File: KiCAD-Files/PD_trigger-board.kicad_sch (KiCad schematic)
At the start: 25 parts, among them J1 USB_C_Receptacle_USB2.0_14P, J10 15V, J11 18V, J2 Conn_01x03, J3 Conn_01x03, J4 VOUT, J5 5V, J6 5V, J7 5V, J8 9V, J9 12V, Q1 AONR21307, U1 HUSB238

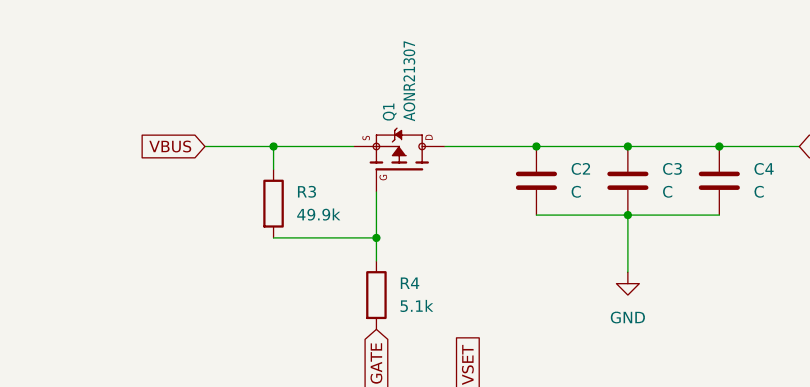
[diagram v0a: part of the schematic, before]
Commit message: Routin fertig
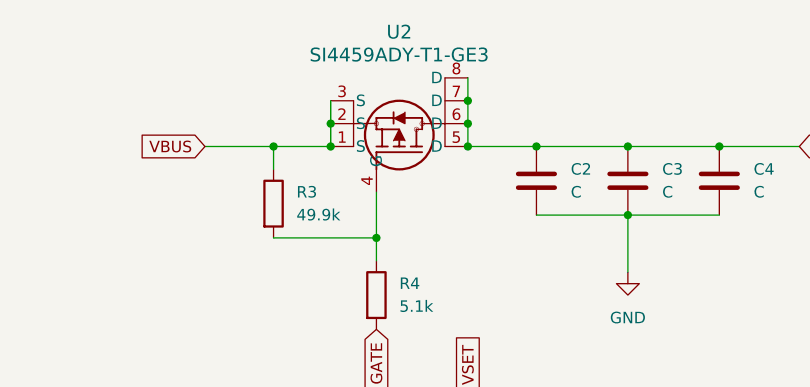
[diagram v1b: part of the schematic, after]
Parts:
- removed Q1: AONR21307, Adafruit HUSB238 USB-C PD Breakout:POWERDI3333, symbol Adafruit HUSB238 USB-C PD Breakout-eagle-import:MOSFET-P-POWERDI3333
- added U2: SI4459ADY-T1-GE3, blinkyparts:SO_ADY-T1-GE3_VIS, symbol SI4459ADY:SI4459ADY-T1-GE3
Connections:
- net VBUS: now also U2.1 (S), U2.2 (S), U2.3 (S)
- net VOUT: now also U2.5 (D), U2.6 (D), U2.7 (D), U2.8 (D)
- net at R3.2, R4.1: now also U2.4 (G)
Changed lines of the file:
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@@
 	(paper "A4")
+	(junction
+		(at 236.22 105.41)
+		(diameter 0)
+		(color 0 0 0 0)
+	)
+	(junction
+		(at 236.22 35.56)
+		(diameter 0)
+		(color 0 0 0 0)
+	)
+	(junction
+		(at 274.32 87.63)
+		(diameter 0)
+		(color 0 0 0 0)
+	)
+	(junction
+		(at 254 35.56)
+		(diameter 0)
+		(color 0 0 0 0)
+	)
+	(junction
+		(at 274.32 96.52)
+		(diameter 0)
+		(color 0 0 0 0)
+	)
+	(junction
+		(at 236.22 87.63)
+		(diameter 0)
+		(color 0 0 0 0)
+	)
+	(junction
+		(at 175.26 138.43)
+		(diameter 0)
+		(color 0 0 0 0)
+	)
+	(junction
+		(at 274.32 105.41)
+		(diameter 0)
+		(color 0 0 0 0)
+	)
+	(junction
+		(at 55.88 88.9)
+		(diameter 0)
+		(color 0 0 0 0)
+	)
+	(junction
+		(at 148.59 127)
+		(diameter 0)
+		(color 0 0 0 0)
+	)
+	(junction
+		(at 226.06 45.72)
+		(diameter 0)
+		(color 0 0 0 0)
+	)
+	(junction
+		(at 243.84 35.56)
+		(diameter 0)
+		(color 0 0 0 0)
+	)
 	(junction
 		(at 214.63 35.56)
@@
 	)
 	(junction
-		(at 236.22 105.41)
-		(diameter 0)
-		(color 0 0 0 0)
-	)
-	(junction
-		(at 274.32 87.63)
-		(diameter 0)
-		(color 0 0 0 0)
-	)
-	(junction
-		(at 254 35.56)
-		(diameter 0)
-		(color 0 0 0 0)
-	)
-	(junction
-		(at 274.32 96.52)
-		(diameter 0)
-		(color 0 0 0 0)
-	)
-	(junction
-		(at 236.22 87.63)
-		(diameter 0)
-		(color 0 0 0 0)
-	)
-	(junction
-		(at 175.26 138.43)
-		(diameter 0)
-		(color 0 0 0 0)
-	)
-	(junction
-		(at 274.32 105.41)
-		(diameter 0)
-		(color 0 0 0 0)
-	)
-	(junction
-		(at 55.88 88.9)
-		(diameter 0)
-		(color 0 0 0 0)
-	)
-	(junction
-		(at 148.59 127)
+		(at 220.98 33.02)
 		(diameter 0)
 		(color 0 0 0 0)
@@
 	)
 	(junction
+		(at 236.22 30.48)
+		(diameter 0)
+		(color 0 0 0 0)
+	)
+	(junction
 		(at 264.16 35.56)
 		(diameter 0)
@@
 	)
 	(junction
-		(at 243.84 35.56)
+		(at 220.98 35.56)
 		(diameter 0)
 		(color 0 0 0 0)
@@
 	)
 	(junction
-		(at 226.06 45.72)
+		(at 236.22 33.02)
 		(diameter 0)
 		(color 0 0 0 0)
@@
 	(wire
 		(pts
+			(xy 220.98 33.02) (xy 220.98 35.56)
+		)
+		(stroke
+			(width 0)
+			(type default)
+		)
+	)
+	(wire
+		(pts
 			(xy 255.27 115.57) (xy 274.32 115.57)
 		)
@@
 	(wire
 		(pts
+			(xy 236.22 30.48) (xy 236.22 33.02)
+		)
+		(stroke
+			(width 0)
+			(type default)
+		)
+	)
+	(wire
+		(pts
 			(xy 148.59 120.65) (xy 148.59 127)
 		)
@@
 	(wire
 		(pts
+			(xy 236.22 33.02) (xy 236.22 35.56)
+		)
+		(stroke
+			(width 0)
+			(type default)
+		)
+	)
+	(wire
+		(pts
 			(xy 81.28 152.4) (xy 83.82 152.4)
 		)
@@
 	(wire
 		(pts
+			(xy 220.98 30.48) (xy 220.98 33.02)
+		)
+		(stroke
+			(width 0)
+			(type default)
+		)
+	)
+	(wire
+		(pts
 			(xy 236.22 87.63) (xy 236.22 96.52)
 		)
@@
 	(wire
 		(pts
+			(xy 236.22 27.94) (xy 236.22 30.48)
+		)
+		(stroke
+			(width 0)
+			(type default)
+		)
+	)
+	(wire
+		(pts
 			(xy 246.38 115.57) (xy 252.73 115.57)
 		)
@@
 	(wire
 		(pts
-			(xy 214.63 35.56) (xy 223.52 35.56)
+			(xy 226.06 40.64) (xy 226.06 45.72)
 		)
 		(stroke
@@
 	(wire
 		(pts
-			(xy 233.68 35.56) (xy 243.84 35.56)
-		)
-		(stroke
-			(width 0)
-			(type default)
-		)
-	)
-	(wire
-		(pts
 			(xy 236.22 105.41) (xy 236.22 115.57)
 		)
@@
 	(wire
 		(pts
+			(xy 236.22 35.56) (xy 243.84 35.56)
+		)
+		(stroke
+			(width 0)
+			(type default)
+		)
+	)
+	(wire
+		(pts
 			(xy 274.32 105.41) (xy 274.32 96.52)
 		)
@@
 	(wire
 		(pts
-			(xy 226.06 40.64) (xy 226.06 45.72)
-		)
-		(stroke
-			(width 0)
-			(type default)
-		)
-	)
-	(wire
-		(pts
 			(xy 264.16 35.56) (xy 273.05 35.56)
 		)
@@
 		(pts
 			(xy 130.81 80.01) (xy 130.81 82.55)
+		)
+		(stroke
+			(width 0)
+			(type default)
+		)
+	)
+	(wire
+		(pts
+			(xy 214.63 35.56) (xy 220.98 35.56)
 		)
 		(stroke
@@
 	)
 	(symbol
-		(lib_id "Adafruit HUSB238 USB-C PD Breakout-eagle-import:MOSFET-P-POWERDI3333")
-		(at 228.6 35.56 90)
-		(unit 1)
-		(exclude_from_sim no)
-		(in_bom yes)
-		(on_board yes)
-		(dnp no)
-		(property "Reference" "Q1"
-			(at 228.219 32.766 0)
-			(effects
-				(font
-					(size 1.27 1.0795)
-				)
-				(justify left bottom)
-			)
-		)
-		(property "Value" "AONR21307"
-			(at 230.505 32.766 0)
-			(effects
-				(font
-					(size 1.27 1.0795)
-				)
-				(justify left bottom)
-			)
-		)
-		(property "Footprint" "Adafruit HUSB238 USB-C PD Breakout:POWERDI3333"
-			(at 228.6 35.56 0)
-			(effects
-				(font
-					(size 1.27 1.27)
-				)
-				(hide yes)
-			)
-		)
-		(property "Datasheet" ""
-			(at 228.6 35.56 0)
-			(effects
-				(font
-					(size 1.27 1.27)
-				)
-				(hide yes)
-			)
-		)
-		(property "Description" ""
-			(at 228.6 35.56 0)
-			(effects
-				(font
-					(size 1.27 1.27)
-				)
-				(hide yes)
-			)
-		)
-		(pin "1"
-		)
-		(pin "2"
-		)
-		(pin "3"
-		)
-		(pin "4"
-		)
-		(pin "5678"
-		)
-		(instances
-			(project "PD_trigger-board"
-				(path "/e428d426-38f9-47e3-9715-a18ed772a1ec"
-					(reference "Q1")
-					(unit 1)
-				)
-			)
-		)
-	)
-	(symbol
 		(lib_id "power:GND")
 		(at 85.09 184.15 0)
@@
 					(unit 1)
 				)
+			)
+		)
+	)
+	(symbol
+		(lib_id "SI4459ADY:SI4459ADY-T1-GE3")
+		(at 226.06 40.64 90)
+		(unit 1)
+		(exclude_from_sim no)
+		(in_bom yes)
+		(on_board yes)
+		(dnp no)
+		(fields_autoplaced yes)
+		(property "Reference" "U2"
+			(at 228.6 22.86 90)
+			(effects
+				(font
+					(size 1.524 1.524)
+				)
+			)
+		)
+		(property "Value" "SI4459ADY-T1-GE3"
+			(at 228.6 25.4 90)
+			(effects
+				(font
+					(size 1.524 1.524)
+				)
+			)
+		)
+		(property "Footprint" "blinkyparts:SO_ADY-T1-GE3_VIS"
+			(at 226.06 40.64 0)
+			(effects
+				(font
+					(size 1.27 1.27)
+					(italic yes)
+				)
+				(hide yes)
+			)
+		)
+		(property "Datasheet" "SI4459ADY-T1-GE3"
+			(at 226.06 40.64 0)
+			(effects
+				(font
+					(size 1.27 1.27)
+					(italic yes)
+				)
+				(hide yes)
+			)
+		)
+		(property "Description" ""
+			(at 226.06 40.64 0)
+			(effects
+				(font
+					(size 1.27 1.27)
+				)
+				(hide yes)
+			)
+		)
+		(pin "2"
+		)
+		(pin "4"
+		)
+		(pin "1"
+		)
+		(pin "7"
+		)
+		(pin "6"
+		)
+		(pin "5"
+		)
+		(pin "3"
+		)
+		(pin "8"
+		)
+		(instances
+			(project ""
+				(path "/e428d426-38f9-47e3-9715-a18ed772a1ec"
+					(reference "U2")
+					(unit 1)
+				)
